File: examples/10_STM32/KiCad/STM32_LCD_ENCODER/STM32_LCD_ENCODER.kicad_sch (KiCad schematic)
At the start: 13 parts, among them J1 Audio In, SW1 ENCODER, U1 STM32F103C6Tx, U2 LCD16X2

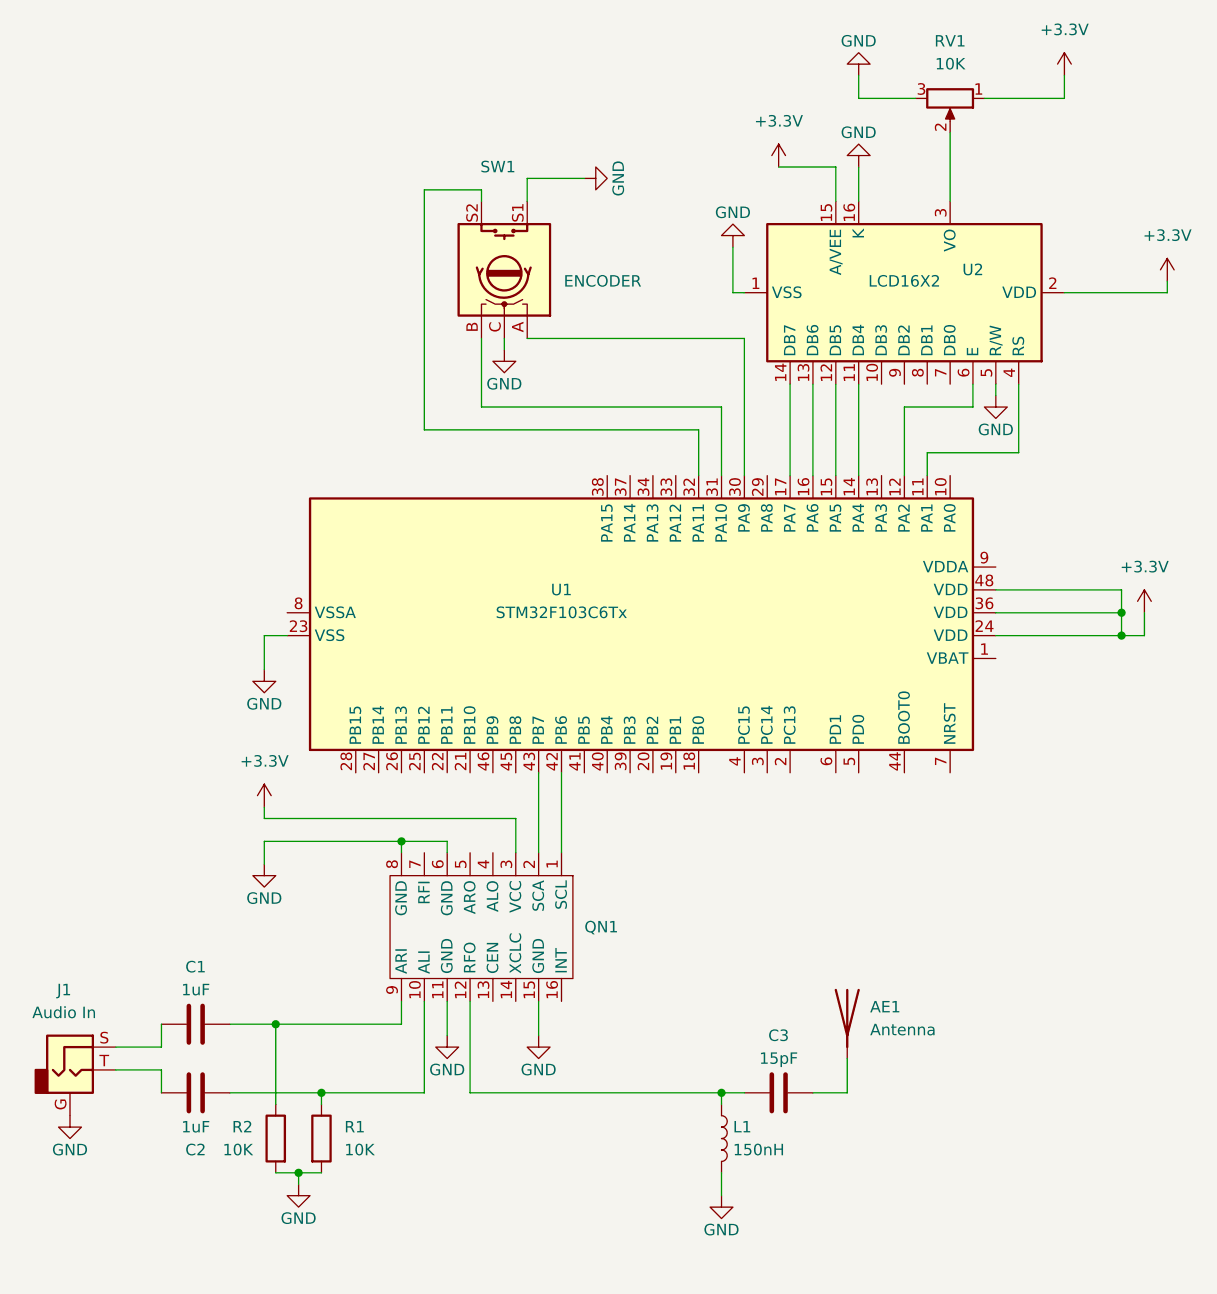
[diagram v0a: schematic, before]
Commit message: Doc
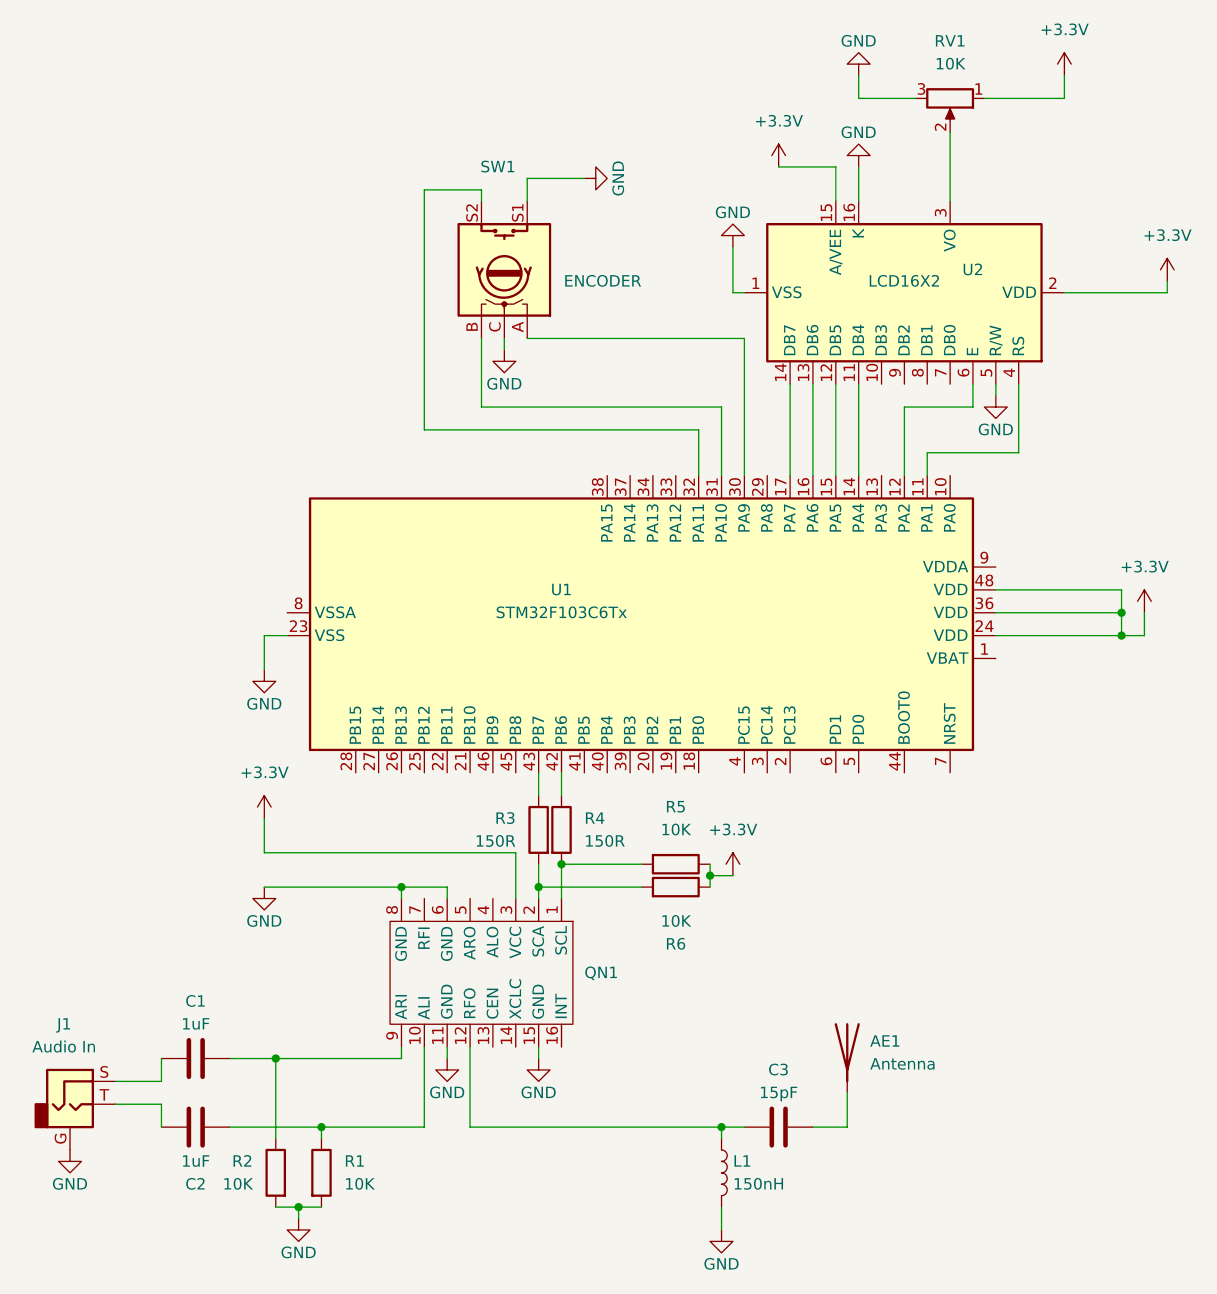
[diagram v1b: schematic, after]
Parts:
- added R3, R4: 150R, symbol Device:R
- added R5, R6: 10K, symbol Device:R
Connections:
- net +3.3V: now also R5.1, R6.1
- net at QN1.1 (SCL): now also R4.2, R5.2; no longer U1.42 (PB6)
- net at U1.43 (PB7): now also R3.1; no longer QN1.2 (SCA)
- new net: QN1.2 (SCA), R3.2, R6.2
- new net: R4.1, U1.42 (PB6)
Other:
- moved on the sheet: AE1, C1, C2, C3, J1, L1, QN1, R1, R2
